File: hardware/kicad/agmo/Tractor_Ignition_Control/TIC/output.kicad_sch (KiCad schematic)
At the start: 40 parts, among them J2 Screw_Terminal_01x06, K1 G5V-2-H1, K2 G5V-2-H1, K3 G5V-2-H1, K4 G5V-2-H1, Q1 IRLML6344, Q5 IRLML6344, Q6 IRLML6344, Q7 IRLML6344, U18 π140U31

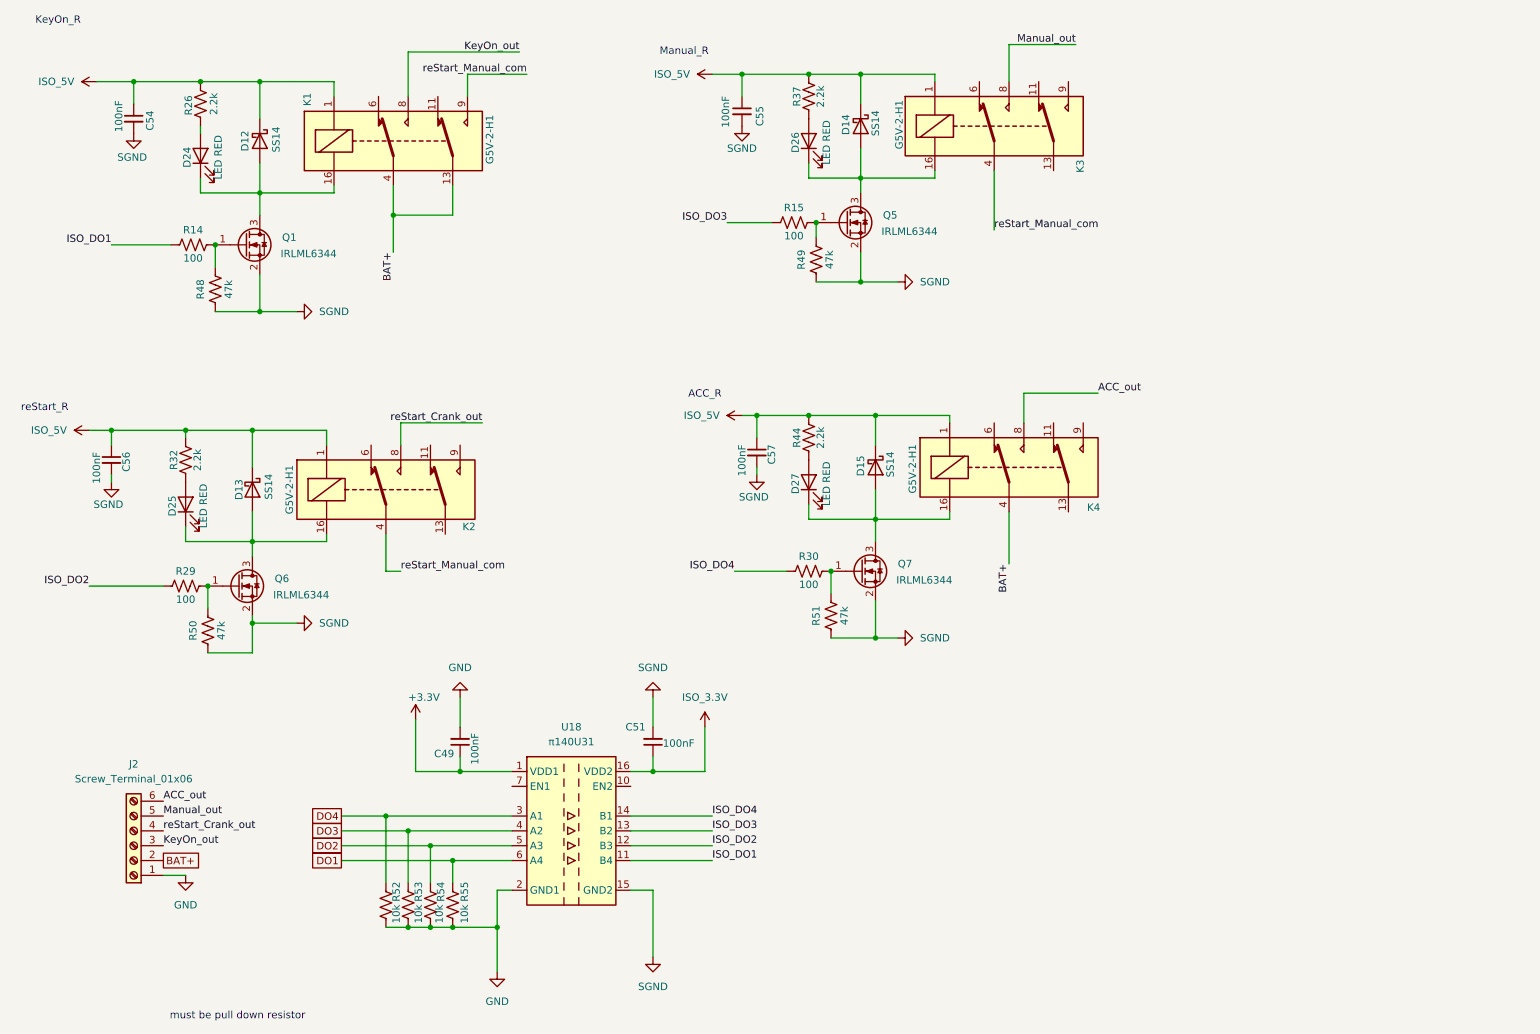
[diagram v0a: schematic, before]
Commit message: feat(hardware): update TIC KiCad design and fabrication files
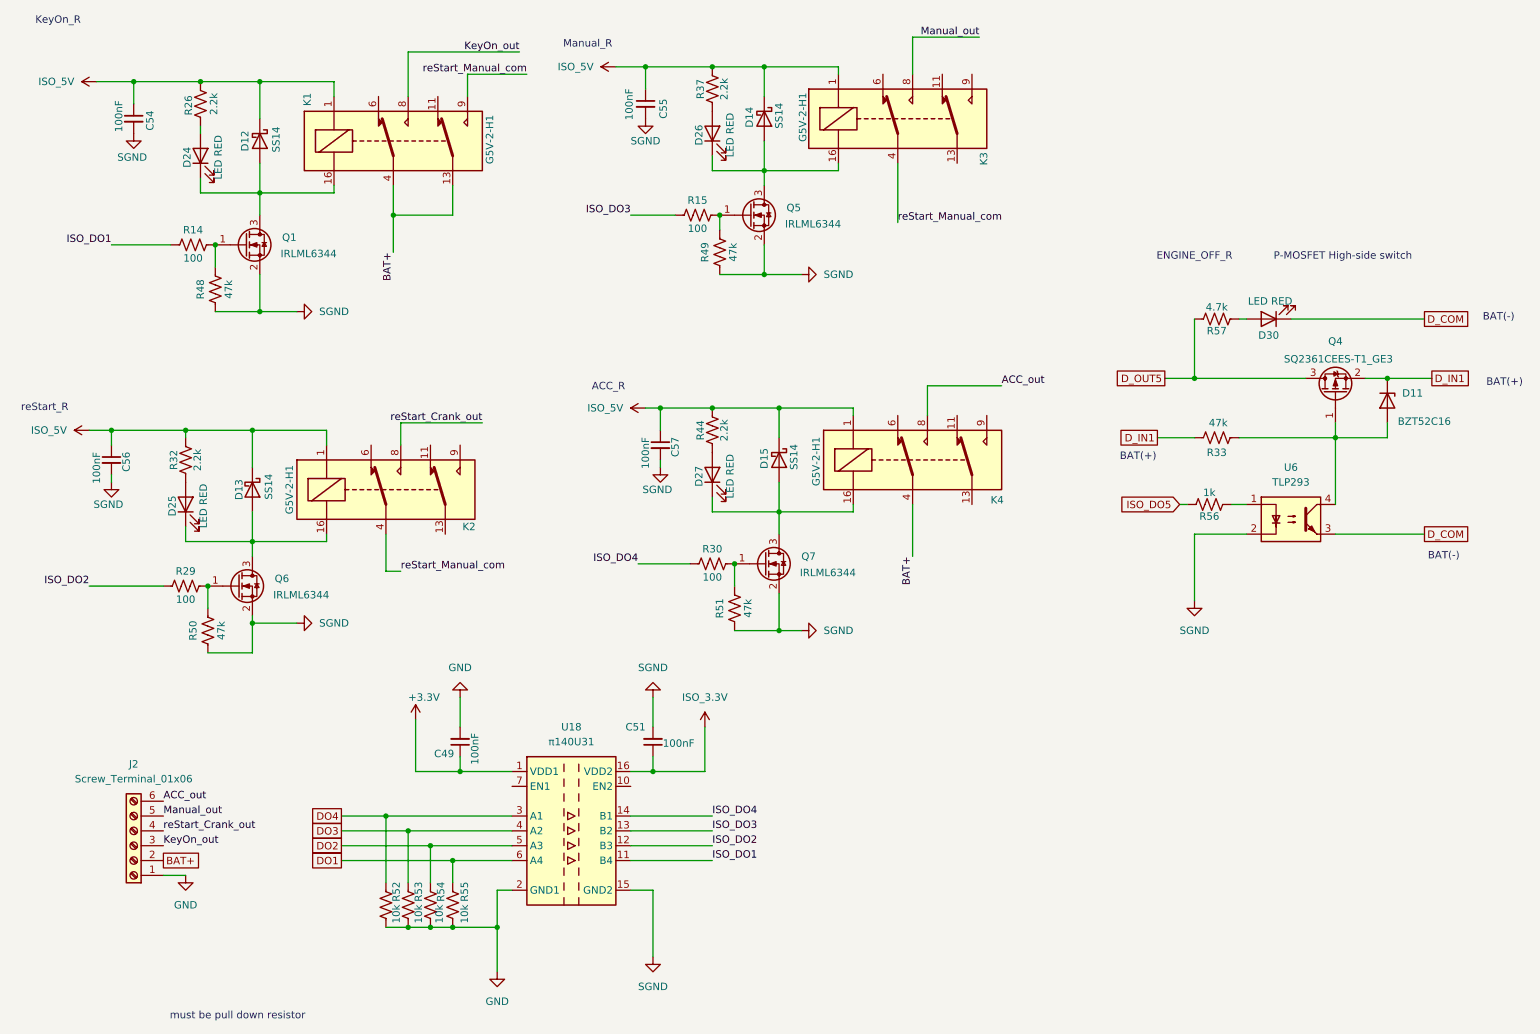
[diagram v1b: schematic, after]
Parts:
- added D11: BZT52C16, Diode_SMD:D_SOD-123, symbol Diode:BZV55C16
- added D30: LED RED, LED_SMD:LED_0805_2012Metric, symbol Device:LED
- added Q4: SQ2361CEES-T1_GE3, Package_TO_SOT_SMD:SOT-23, symbol Transistor_FET:IRLML5203
- added R33: 47k, Resistor_SMD:R_0805_2012Metric, symbol Device:R_US
- added R56: 1k, Resistor_SMD:R_0805_2012Metric, symbol Device:R_US
- added R57: 4.7k, Resistor_SMD:R_0805_2012Metric, symbol Device:R_US
- added U6: TLP293, Package_SO:SOIC-4_4.55x2.6mm_P1.27mm, symbol Isolator:TLP293
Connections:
- net SGND: now also U6.2
- new net: D11.2 (A), Q4.1 (G), R33.1, U6.4
- new net: R56.2, U6.1
- new net: D30.2 (A), R57.2
- new net D_COM: D30.1 (K), U6.3
- new net D_IN1: D11.1 (K), Q4.2 (S), R33.2
- new net D_OUT5: Q4.3 (D), R57.1
- new net ISO_DO5: R56.1
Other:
- note added: "BAT(+)"
- note added: "BAT(-)"
- note added: "ENGINE_OFF_R"
- note added: "P-MOSFET High-side switch"
- moved on the sheet: C55, C57, D14, D15, D26, D27, K3, K4, Q5, Q7, R15, R30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
